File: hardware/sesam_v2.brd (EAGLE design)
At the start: 70 x 70 mm, 11 parts, among them X2 C-GRID-06-70543

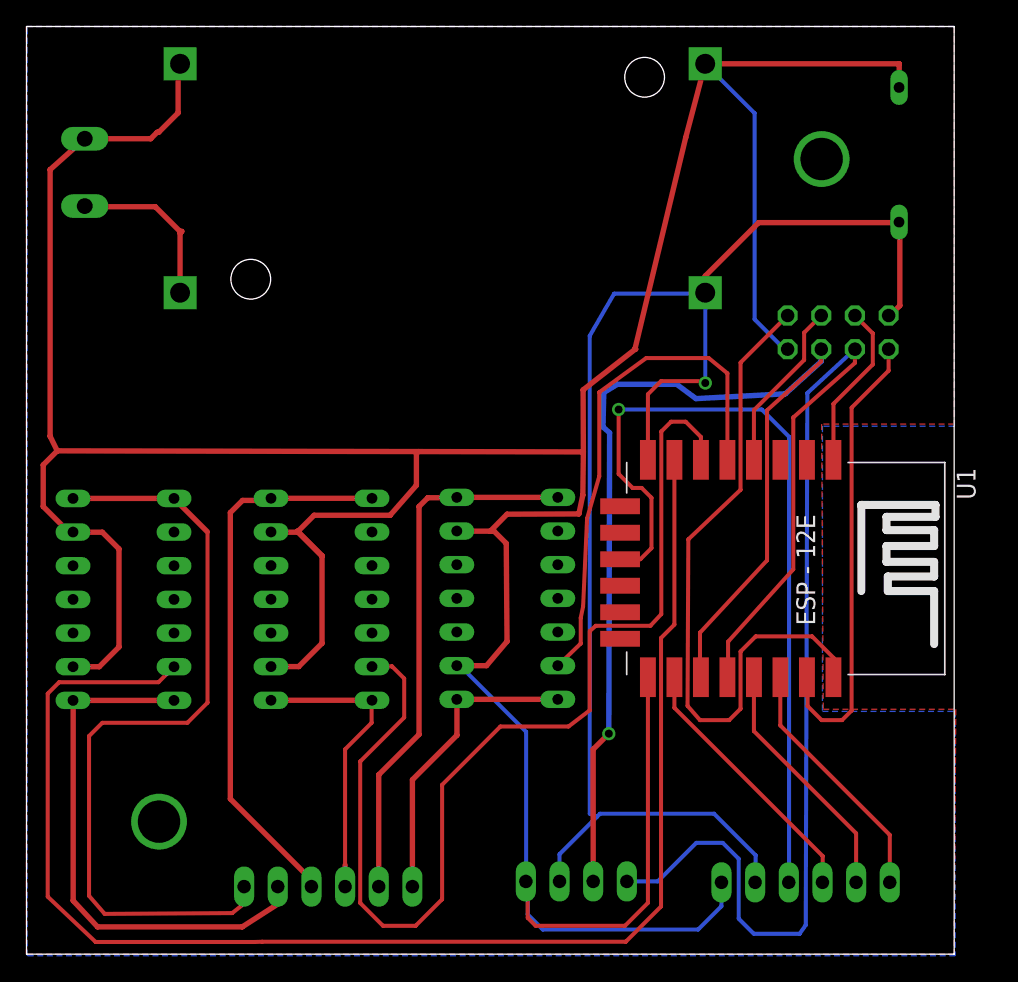
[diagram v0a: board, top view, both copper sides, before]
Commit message: new nice layout
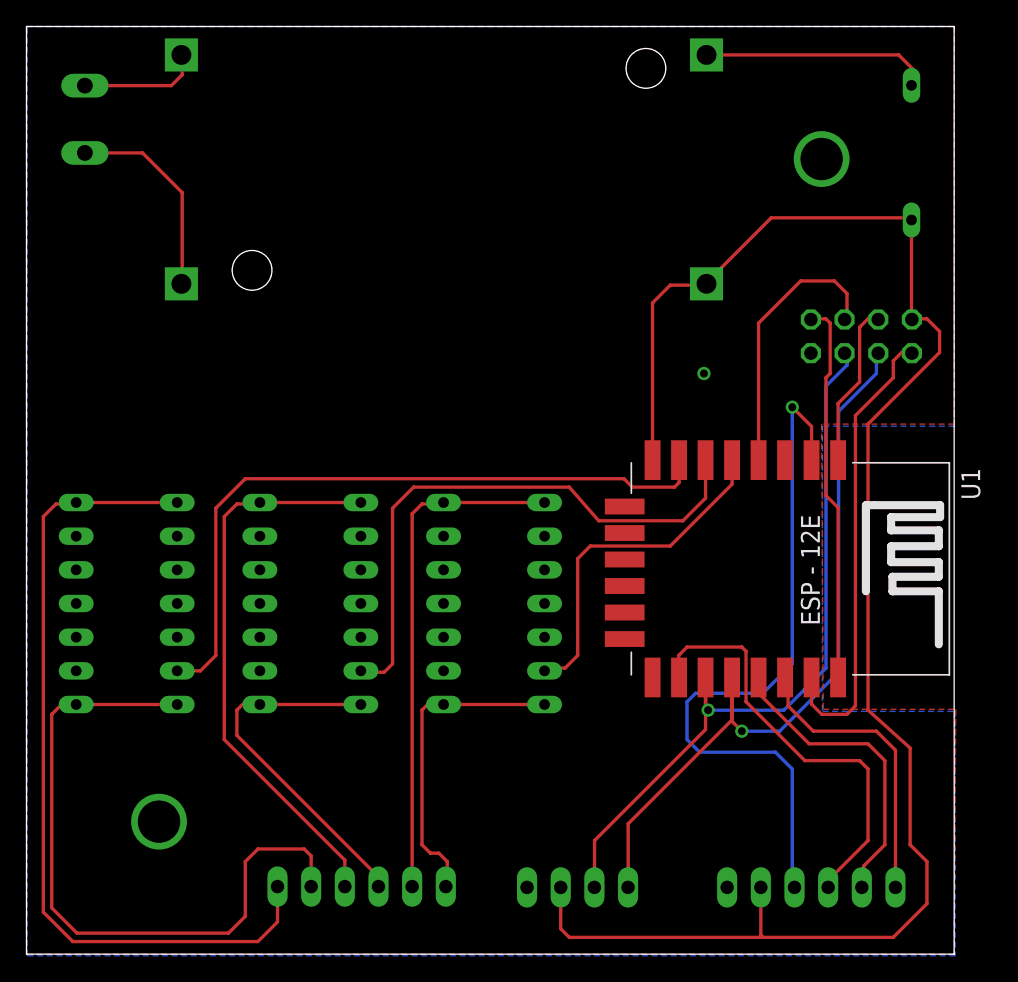
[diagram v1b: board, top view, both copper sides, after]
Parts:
- moved X1 4.01 mm to (5.04, 63.0)
- moved OUTPUT_CON 2.52 mm to (25.3, 5.10)
- moved SERIAL 1.78 mm to (63.0, 46.6)
- moved RELAIS_3 1.07 mm to (35.3, 26.5)
- moved D1 0.95 mm to (66.8, 60.5)
- moved RELAIS_2 0.90 mm to (21.4, 26.5)
- moved U$1 0.68 mm to (31.5, 59.2)
- moved X2 0.57 mm to (59.2, 5.04)
- moved OLED 0.46 mm to (41.6, 5.04)
- moved RELAIS_1 0.39 mm to (7.56, 26.5)
- moved U1 0.35 mm to (55.4, 29.0)
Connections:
- net N$12: now also U1.ADC; no longer U1.GPIO9
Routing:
- net GND: track 300.2 -> 26.6 mm, vias 0 -> 1
- net N$13: track 108.6 -> 52.5 mm
- net N$14: track 82.1 -> 43.5 mm
- net N$16: track 94.3 -> 57.9 mm, vias 0 -> 1
- net N$21: track 85.0 -> 56.6 mm
- net N$17: track 51.4 -> 28.9 mm
- net 3V3: track 110.3 -> 127.5 mm, vias 1 -> 0
- net N$15: track 39.0 -> 26.1 mm
- net N$11: track 20.1 -> 32.4 mm
- net N$4: track 41.1 -> 52.5 mm
- net N$12: track 61.9 -> 53.8 mm
- net N$18: track 13.0 -> 20.8 mm
- net N$6: track 22.5 -> 27.4 mm
- net N$10: track 18.7 -> 23.1 mm
- net N$9: track 18.9 -> 22.1 mm
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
